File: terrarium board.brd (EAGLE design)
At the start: 100 x 100.3 mm, 30 parts

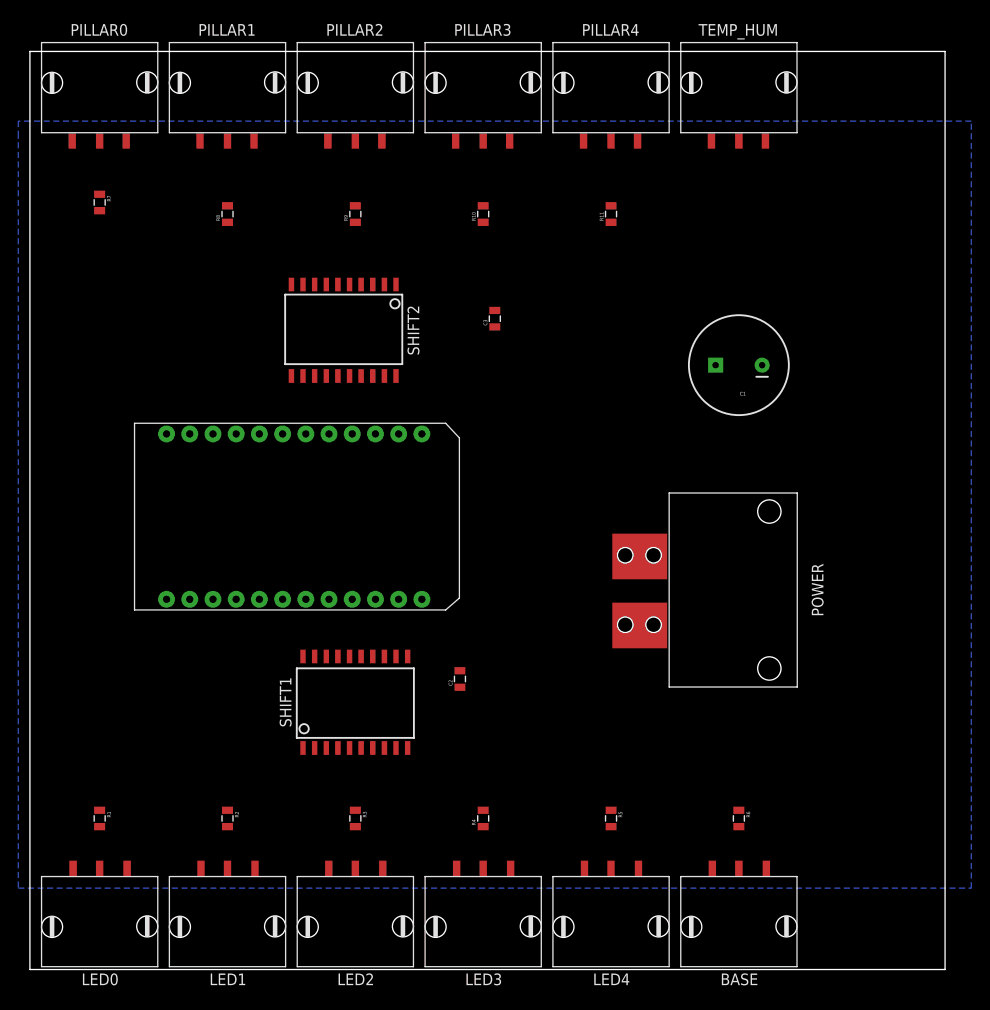
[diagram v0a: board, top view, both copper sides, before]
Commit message: Getting ready to send v2 to OSH Park.
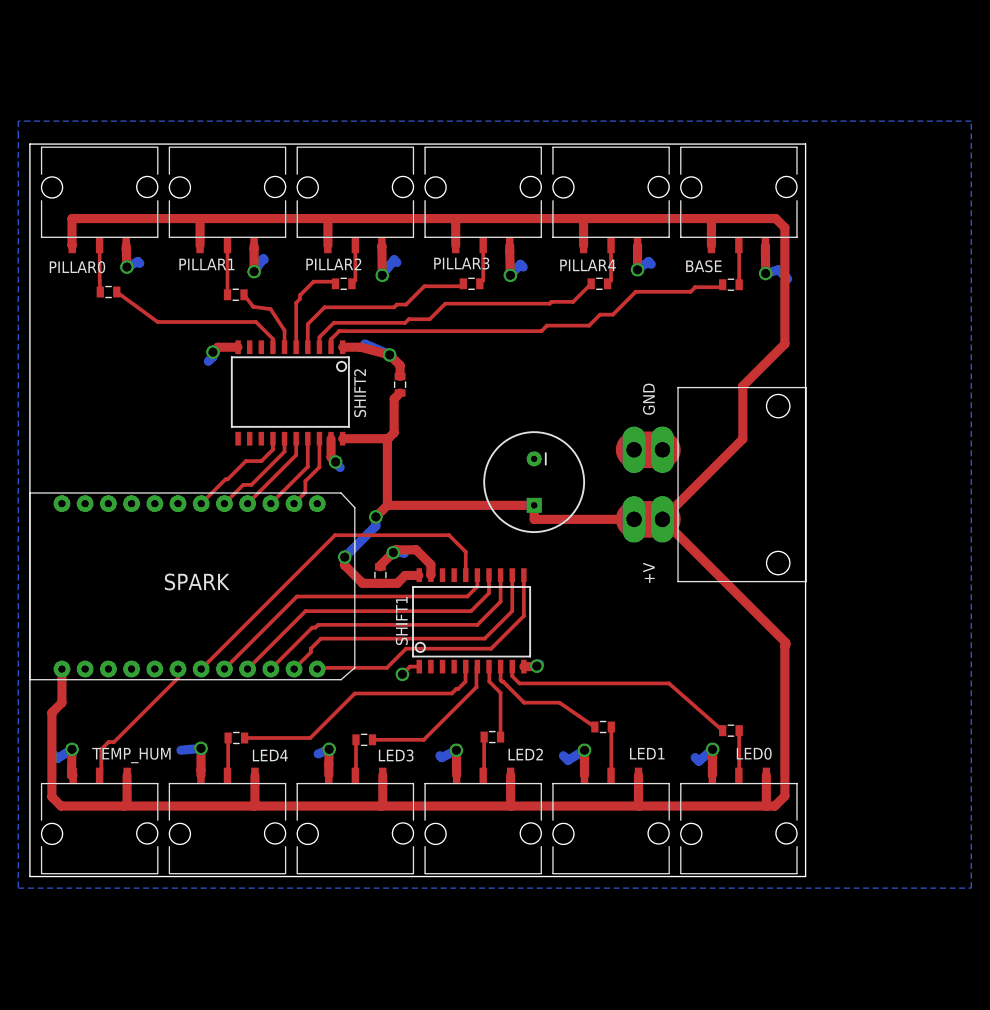
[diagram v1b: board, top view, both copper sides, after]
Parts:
- moved TEMP_HUM 91.2 mm to (14.0, 10.2), turned to 180 degrees
- moved BASE 71.0 mm to (71.1, 69.8), turned to 0 degrees
- moved LED0 70.6 mm to (83.8, 10.2)
- moved R1 69.6 mm to (76.6, 15.9), turned to 0 degrees
- moved R6 58.3 mm to (76.6, 64.7), turned to 0 degrees
- moved LED1 43.1 mm to (69.8, 10.2)
- moved LED4 43.1 mm to (27.9, 10.2)
- moved R2 42.2 mm to (62.6, 16.3), turned to 0 degrees
- moved R5 41.9 mm to (22.6, 15.1), turned to 180 degrees
- moved C1 25.8 mm to (55.1, 43.1), turned to 270 degrees
- moved R3 17.4 mm to (50.5, 15.2), turned to 180 degrees
- moved LED2 17.3 mm to (55.9, 10.2)
- moved LED3 17.3 mm to (41.9, 10.2)
- moved R4 15.6 mm to (36.5, 14.9), turned to 180 degrees
- moved SHIFT1 15.5 mm to (48.3, 27.9)
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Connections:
- removed net N$1: C3.1, SHIFT2.20
- removed net N$27: R8.1, SHIFT2.5
- removed net N$28: R7.1, SHIFT2.6
- removed net N$29: SPARK.D0, TEMP_HUM.DIN
- new net N$10: R6.1, SHIFT2.2
- new net N$12: SPARK.A6, TEMP_HUM.DIN
- new net N$13: R11.1, SHIFT2.3
- new net N$15: R10.1, SHIFT2.4
- net +5V: now also C3.1, POWER.VCC1, POWER.VCC2, SHIFT2.20; no longer POWER.VCC
- net GND: now also POWER.GND1, POWER.GND2; no longer POWER.GND
- net N$23: now also R9.1, SHIFT2.5; no longer R6.1, SHIFT1.4
- net N$24: now also R8.1, SHIFT2.6; no longer R11.1, SHIFT2.2
- net N$25: now also R7.1, SHIFT2.7; no longer R10.1, SHIFT2.3
- net N$26: now also SHIFT2.13; no longer R9.1, SHIFT2.4
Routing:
- net +5V: track 0.00 -> 357.5 mm, vias 0 -> 2
- net GND: track 0.00 -> 96.7 mm, vias 0 -> 18
- net N$10: track 0.00 -> 46.1 mm
- net N$39: track 0.00 -> 38.3 mm
- net N$13: track 0.00 -> 33.2 mm
- net N$38: track 0.00 -> 32.6 mm
- net N$37: track 0.00 -> 31.8 mm
- net N$36: track 0.00 -> 31.1 mm
- net N$35: track 0.00 -> 30.6 mm
- net N$34: track 0.00 -> 29.4 mm
- net N$22: track 0.00 -> 28.3 mm
- net N$5: track 0.00 -> 26.3 mm
- net N$15: track 0.00 -> 21.3 mm
- net N$25: track 0.00 -> 19.8 mm
- net N$21: track 0.00 -> 16.0 mm
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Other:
- board size 100 x 100.3 mm -> 84.8 x 80 mm
- board text added: "SPARK"
